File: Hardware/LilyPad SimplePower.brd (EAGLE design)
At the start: 10.2 x 30.5 mm, 11 parts

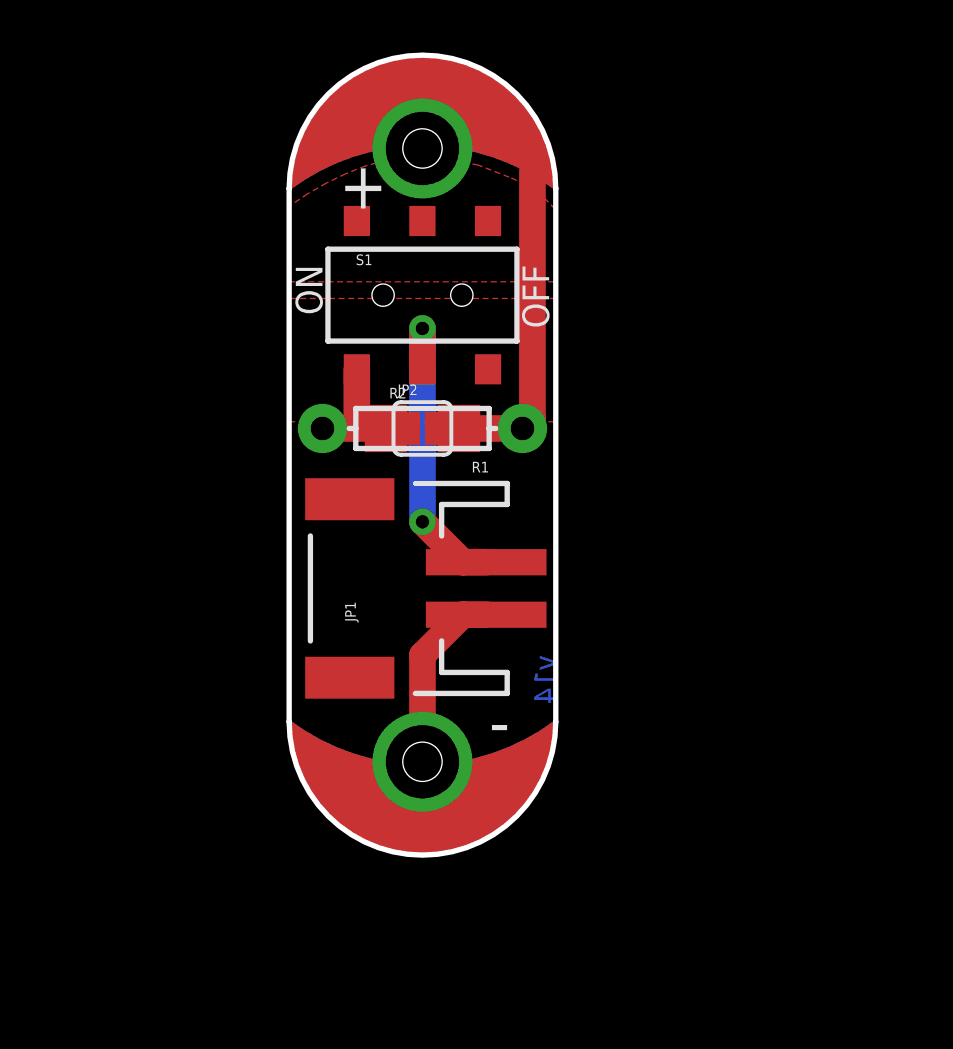
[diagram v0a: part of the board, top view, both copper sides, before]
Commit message: Hardware Version 2.0 commit
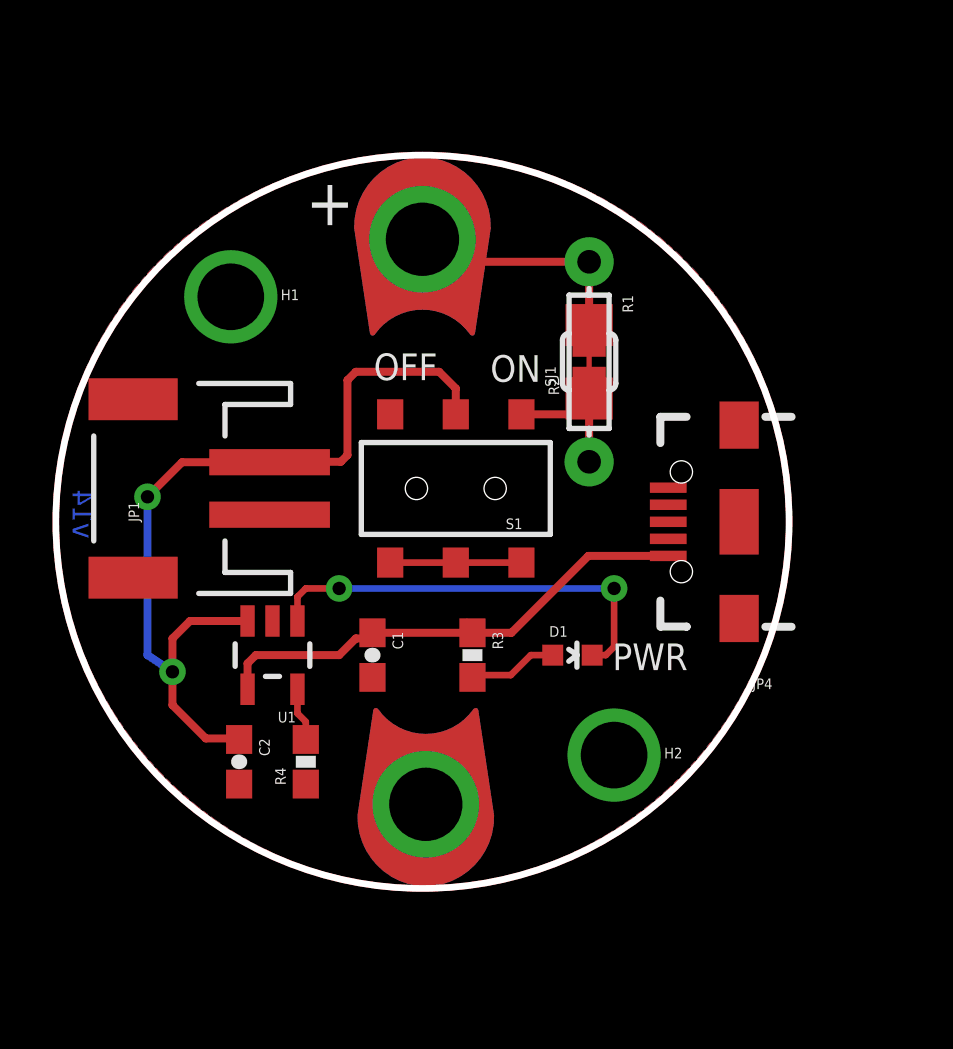
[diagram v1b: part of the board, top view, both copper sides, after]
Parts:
- removed JP2: (no value), SparkFun-Passives:SJ_2S
- added C1, C2: 4.7uF, SparkFun-Capacitors:0603-CAP
- added D1: (no value), SparkFun-LED:LED-0603
- added H1, H2: SEW_HOLE, LilyPad-Wearables:SIMPLE_HOLE
- added JP4: USB_MICROB_PLUGCONN-11752, SparkFun-Connectors:USB-B-MICRO-SMD_V03
- added R3: 330, SparkFun-Resistors:0603-RES
- added R4: 2.0k, SparkFun-Resistors:0603-RES
- added SJ1: SOLDERJUMPERTRACE, SparkFun-Passives:SJ_2S-TRACE
- added U1: MCP73831, SparkFun-PowerIC:SOT23-5
- U$3, U$4: value SEWTAP7 -> SEWTAP9; device LilyPad-Wearables:PETAL-LARGE-2SIDE -> LilyPad-Wearables:PETAL-LONG-1-2SIDE
- moved JP3 17.0 mm to (6.35, -7.30), turned to 0 degrees
- moved JP1 9.09 mm to (-9.53, -1.27)
- moved S1 7.47 mm to (1.27, -1.27), turned to 180 degrees
- moved U$4 6.98 mm to (0.00, 8.26), turned to 270 degrees
- moved R1 6.84 mm to (6.35, 3.56), turned to 270 degrees
- moved R2 6.84 mm to (6.35, 3.56), turned to 90 degrees
- moved U$5 6.33 mm to (-6.03, -5.71), turned to 0 degrees
- moved U$3 1.91 mm to (0.13, -13.3), turned to 90 degrees
- moved U$1 1.42 mm to (-0.64, 1.27), turned to 180 degrees
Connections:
- new net N$3: C1.1, JP4.VBUS1, R3.1, U1.4
- new net N$4: D1.C, U1.1
- new net N$5: D1.A, R3.2
- new net N$7: R4.2, U1.5
- net +: now also SJ1.2; no longer JP2.2
- net GND: now also C1.2, C2.2, JP4.GND1, R4.1, U1.2
- net N$1: now also C2.1, U1.3
- net N$2: now also SJ1.1; no longer JP2.1
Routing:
- net N$1: track 12.0 -> 32.6 mm
- net N$3: track 0.00 -> 19.2 mm
- net N$4: track 0.00 -> 16.3 mm, vias 0 -> 2
- net +: track 19.1 -> 10.0 mm
- net GND: track 7.13 -> 0.00 mm
- net SINK1: track 0.00 -> 5.30 mm
- net N$5: track 0.00 -> 3.41 mm
- net N$7: track 0.00 -> 2.05 mm
- added copper zone on layer 1, net GND
- added copper zone on layer 16, net GND
- removed copper zone on layer 1, net SINK1
- removed copper zone on layer 1, net SINK2
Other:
- board size 10.2 x 30.5 mm -> 27.9 x 27.9 mm
- board text added: "PWR"
- board text removed: "-"
